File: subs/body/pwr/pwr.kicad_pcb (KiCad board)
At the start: 2 copper layers, 12.5 x 25.5 mm, 2 parts, among them P1 CON_BAT_IN, P2 CON_BAT_OUT

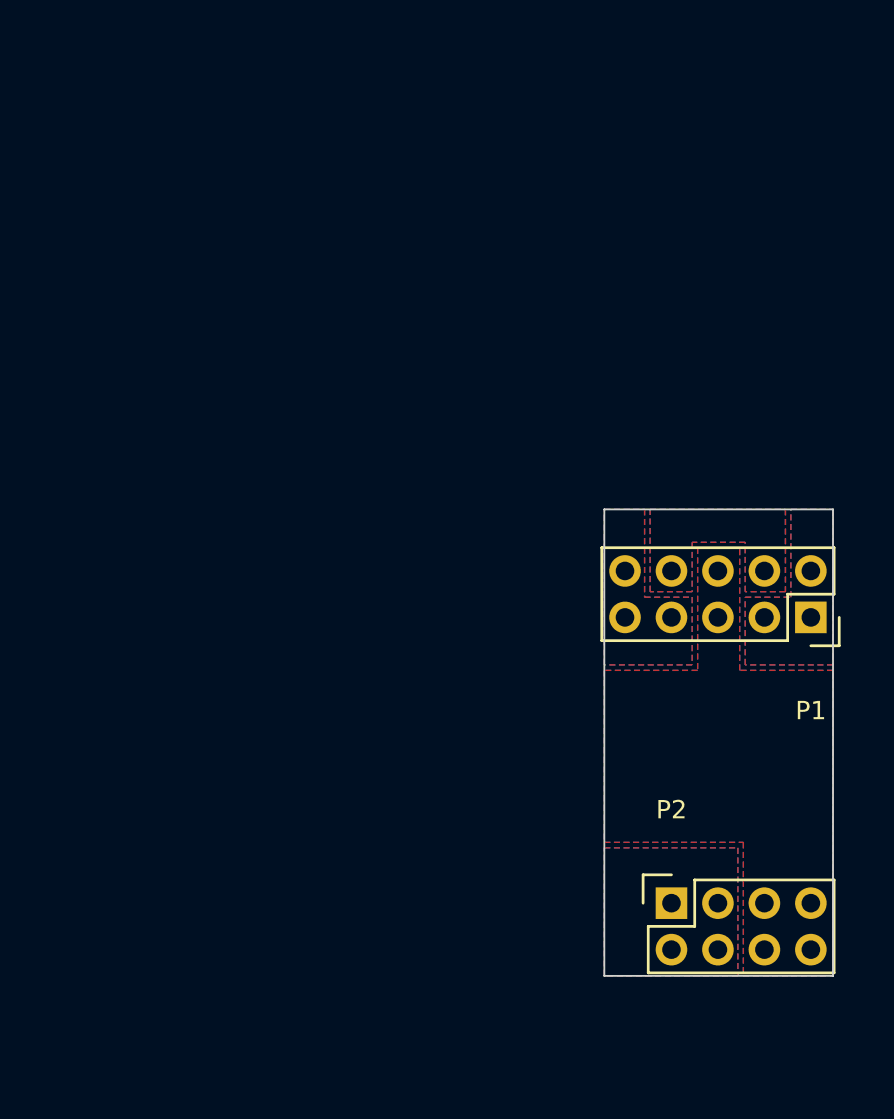
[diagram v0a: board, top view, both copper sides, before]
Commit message: Major modification of body board and companions
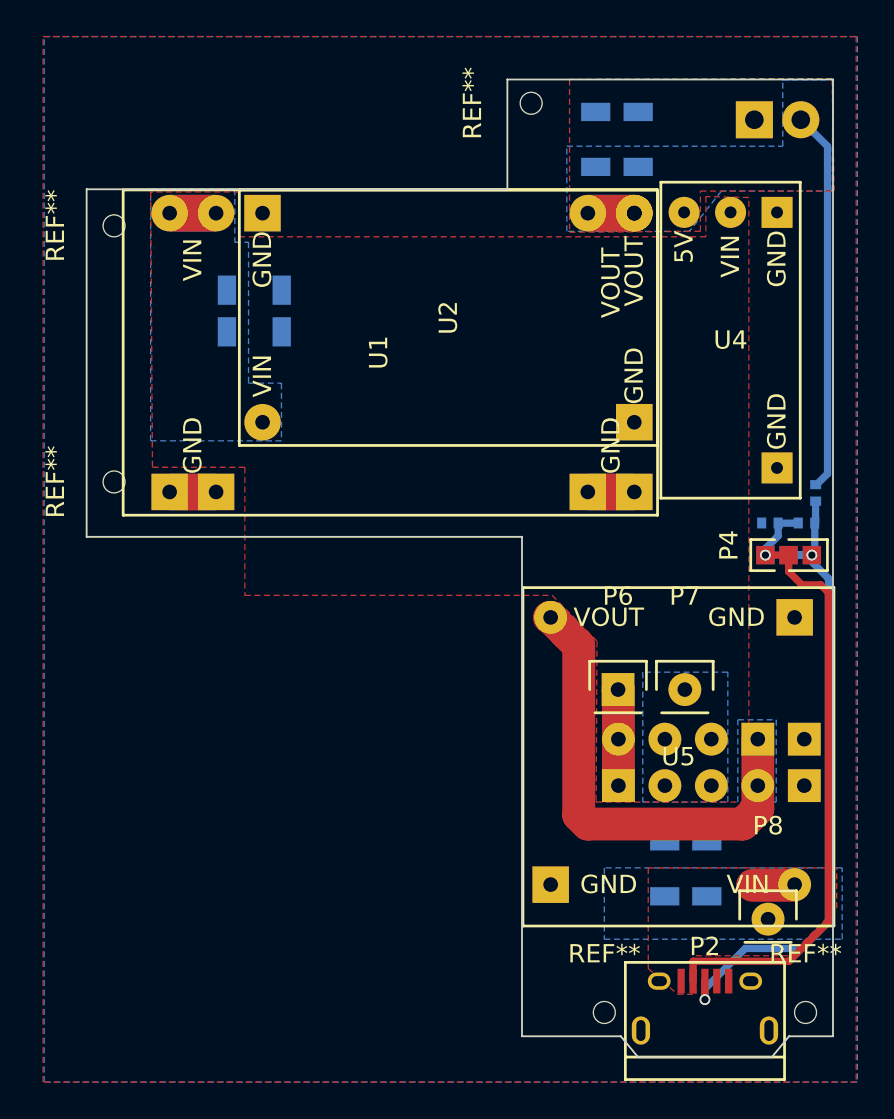
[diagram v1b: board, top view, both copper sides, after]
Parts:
- added C1: 47uF, Capacitors_SMD:C_1206, B.Cu at (67.4, 111.0)
- added C2: 47uF, Capacitors_SMD:C_1206, B.Cu at (89.8, 142.7)
- added C3: 47uF, Capacitors_SMD:C_1206, B.Cu at (86.0, 102.8)
- added C4: 47uF, Capacitors_SMD:C_1206, B.Cu at (92.1, 142.7)
- added C5: 47uF, Capacitors_SMD:C_1206, B.Cu at (67.4, 113.3)
- added C6: 47uF, Capacitors_SMD:C_1206, B.Cu at (88.3, 102.8)
- added P3: CONN_VCC, Socket_Strips:Socket_Strip_Straight_1x02, B.Cu at (94.7, 101.7)
- added P4: CONN_01X03, Pin_Headers:Pin_Header_Straight_1x03_Pitch1.27mm, F.Cu at (95.3, 125.5)
- added P5: CONN_01X03, Pin_Headers:Pin_Header_Straight_1x03_Pitch1.27mm, B.Cu at (95.3, 125.5)
- added P6: CONN_01X01, Pin_Headers:Pin_Header_Straight_1x01, F.Cu at (87.2, 132.8)
- added P7: CONN_01X01, Pin_Headers:Pin_Header_Straight_1x01, F.Cu at (90.9, 132.8)
- added P8: CONN_01X01, Pin_Headers:Pin_Header_Straight_1x01, F.Cu at (95.5, 145.4)
- added R1: 2M, Resistors_SMD:R_0402, B.Cu at (98.0, 122.1)
- added R2: 1M, Resistors_SMD:R_0402, B.Cu at (97.5, 123.8)
- added R3: 400K, Resistors_SMD:R_0402, B.Cu at (95.5, 123.8)
- added REF**: MountingHole_1.2mm_M1, Mounting_Holes:MountingHole_1.2mm_M1, F.Cu at (82.5, 100.8)
- added REF**: MountingHole_1.2mm_M1, Mounting_Holes:MountingHole_1.2mm_M1, F.Cu at (59.7, 121.5)
- added REF**: MountingHole_1.2mm_M1, Mounting_Holes:MountingHole_1.2mm_M1, F.Cu at (59.7, 107.5)
- added REF**: MountingHole_1.2mm_M1, Mounting_Holes:MountingHole_1.2mm_M1, F.Cu at (86.5, 150.5)
- added REF**: MountingHole_1.2mm_M1, Mounting_Holes:MountingHole_1.2mm_M1, F.Cu at (97.5, 150.5)
- added U1: TPS61800 module, Converters_DCDC_ACDC:DCDC_Conv_TPS61800-Boost, F.Cu at (74.2, 114.4)
- added U2: G5177 module, Converters_DCDC_ACDC:DCDC_Conv_G5177-Boost, F.Cu at (78.0, 112.5)
- added U4: LDO_3V5, Converters_DCDC_ACDC:LDO_RT9018, F.Cu at (93.4, 113.8)
- added U5: TP5000 Charger, Converters_DCDC_ACDC:DCDC_Charger-TP5000-Bucket, F.Cu at (90.6, 136.5)
- P1: value CON_BAT_IN -> CONN5; moved to B.Cu
- P2: value CON_BAT_OUT -> USB_Micro; footprint Socket_Strips:Socket_Strip_Straight_2x04 -> Connect:USB_Micro-B
- moved P1 14.0 mm to (87.3, 138.1), turned to 0 degrees
- moved P2 6.10 mm to (92.0, 150.3)
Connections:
- P1 pad 1: /BAT_VIN2 -> GND
- P1 pad 10: /BAT_VIN1 -> GND
- P1 pad 2: /BAT_VIN2 -> GND
- P1 pad 3: /BAT_VIN2 -> /BAT
- P1 pad 4: /CHARGE -> /BAT
- P1 pad 5: /GND -> /BAT
- P1 pad 6: /GND -> /BAT
- P1 pad 7: /BAT_VIN1 -> /CHARGE
- P1 pad 9: /BAT_VIN1 -> GND
- P2 pad 1: /BAT -> /CHG_IN
- P2 pad 2: /BAT -> /V0.6
- P2 pad 3: /BAT -> /V3.3
- P2 pad 4: /BAT -> (no net)
- P2 pad 5: /GND -> GND
- P2 pad 6: /GND -> GND
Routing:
- net /V3.3: track 0.00 -> 35.9 mm, vias 0 -> 2
- net /V0.6: track 0.00 -> 35.3 mm, vias 0 -> 1
- net /CHARGE: track 0.00 -> 25.7 mm
- net VCC: track 0.00 -> 21.8 mm
- net GND: track 0.00 -> 5.26 mm
- net /CHG_IN: track 0.00 -> 2.37 mm
- added copper zone on B.Cu, net /CHG_IN
- added copper zone on F.Cu, net /CHG_IN
- added copper zone on B.Cu, net GND
- added copper zone on F.Cu, net GND
- added copper zone on B.Cu, net VCC
- added copper zone on F.Cu, net VCC
- removed copper zone on B.Cu, net /BAT_VIN1
- removed copper zone on F.Cu, net /BAT_VIN1
- removed copper zone on B.Cu, net /BAT_VIN2
- removed copper zone on F.Cu, net /BAT_VIN2
- removed copper zone on F.Cu, net /CHARGE
- removed copper zone on B.Cu, net /GND
- removed copper zone on F.Cu, net /GND
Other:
- board size 12.5 x 25.5 mm -> 40.8 x 53.4 mm
